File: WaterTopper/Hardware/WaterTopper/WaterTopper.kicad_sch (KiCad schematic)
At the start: 60 parts, among them J1 TYPE-C-31-M-12, J2 Barrel_Jack_Switch, J3 Conn_01x07, J4 Conn_01x04, J5 Conn_01x04, J6 Conn_01x04, J7 Conn_01x04, J8 Screw_Terminal_01x02, J9 Screw_Terminal_01x02, SW1 SW_SPST, SW2 SW_SPST, U1 AP2112K-3.3, U2 ESP32-S3-MINI-1-N8, U3 DRV8881PRHRT, U4 BMP280

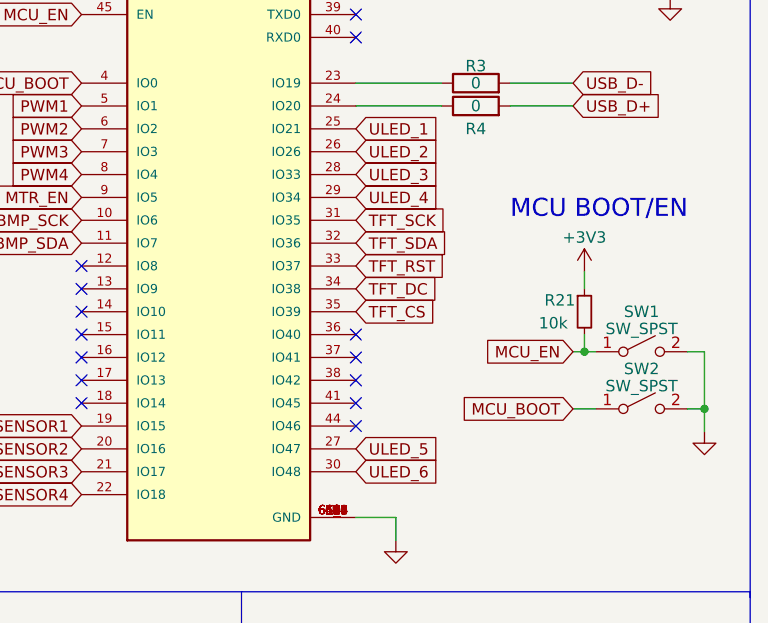
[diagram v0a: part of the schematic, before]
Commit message: Updated pcb design
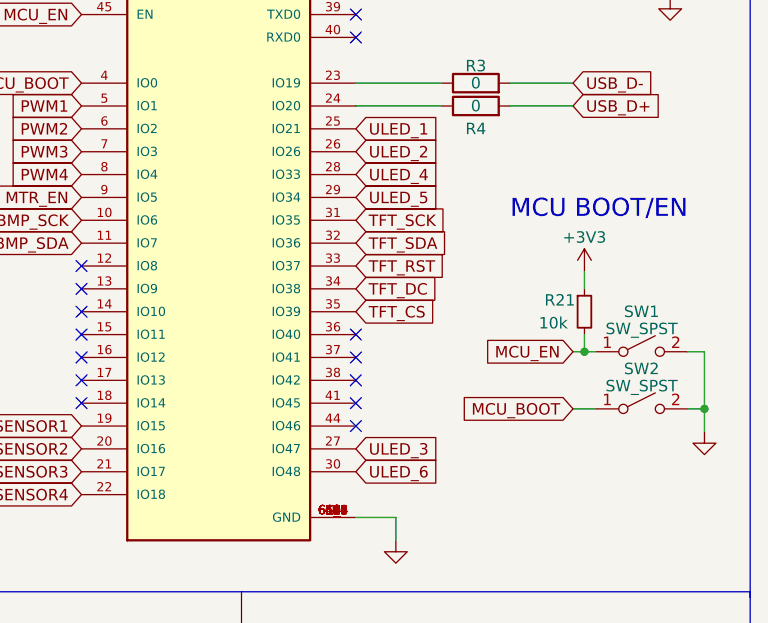
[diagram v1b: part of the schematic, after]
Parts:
- C10, C11, C12, C5, C6, C7, C8, C9: footprint (none) -> Capacitor_SMD:C_01005_0402Metric
- D3, D4, D5, D6, D7, D8: footprint (none) -> LED_SMD:LED_0201_0603Metric
- J4: footprint Connector_JST:JST_XH_S4B-XH-A-1_1x04_P2.50mm_Horizontal -> Connector_JST:JST_PH_B4B-PH-K_1x04_P2.00mm_Vertical
- J5, J6, J7: footprint Connector_JST:JST_XH_S4B-XH-A_1x04_P2.50mm_Horizontal -> Connector_JST:JST_PH_B4B-PH-K_1x04_P2.00mm_Vertical
- R10, R11, R12, R13, R14, R15, R16, R17, R18, R19, R20, R21, R7: footprint (none) -> Resistor_SMD:R_01005_0402Metric
- SW1, SW2: footprint (none) -> Button_Switch_SMD:SW_SPST_PTS810
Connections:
- net ULED_3: now also U2.27 (IO47); no longer U2.28 (IO33)
- net ULED_4: now also U2.28 (IO33); no longer U2.29 (IO34)
- net ULED_5: now also U2.29 (IO34); no longer U2.27 (IO47)

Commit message: Updated pcb + 4 layer
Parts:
- C1: footprint Capacitor_SMD:C_0201_0603Metric -> Capacitor_SMD:C_0805_2012Metric
- C10, C11, C12, C2, C5, C6, C7, C9: footprint Capacitor_SMD:C_01005_0402Metric -> Capacitor_SMD:C_0603_1608Metric
- C3, C4: footprint Capacitor_SMD:C_01005_0402Metric -> Capacitor_SMD:C_0805_2012Metric
- C8: footprint Capacitor_SMD:C_01005_0402Metric -> Capacitor_SMD:C_Elec_6.3x5.8
- D3, D4, D5, D6, D7, D8: footprint LED_SMD:LED_0201_0603Metric -> LED_SMD:LED_0603_1608Metric
- H1, H2, H3, H4: footprint MountingHole:MountingHole_2.7mm_M2.5 -> MountingHole:MountingHole_3.2mm_M3
- R1, R2, R3, R4, R5, R6, R8, R9: footprint Capacitor_SMD:C_01005_0402Metric -> Resistor_SMD:R_0603_1608Metric
- R10, R11, R12, R13, R14, R15, R16, R17, R18, R19, R20, R21, R7: footprint Resistor_SMD:R_01005_0402Metric -> Resistor_SMD:R_0603_1608Metric
